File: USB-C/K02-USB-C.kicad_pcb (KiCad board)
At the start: 2 copper layers, 109.4 x 86.9 mm, 28 parts, among them SW1 SW_Push, SW10 SW_Push, SW11 SW_Push, SW12 SW_Push, SW13 SW_Push, SW14 SW_Push, SW15 SW_Push, SW16 SW_Push, SW17 SW_Push, SW2 SW_Push, SW3 SW_Push, SW4 SW_Push, SW5 SW_Push, SW6 SW_Push, SW7 SW_Push, SW8 SW_Push, SW9 SW_Push, U1 ProMicro-kbd

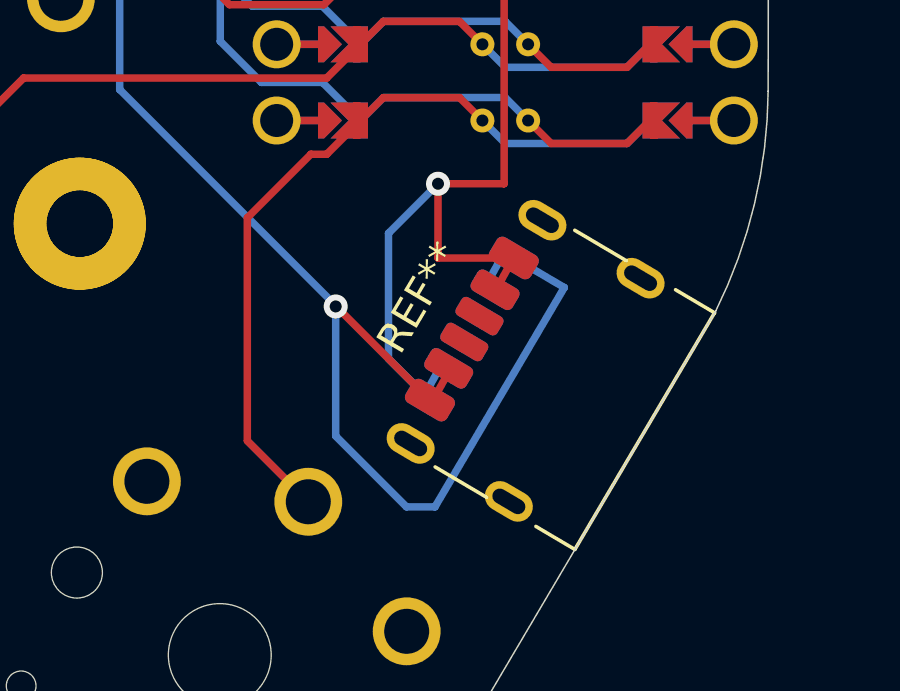
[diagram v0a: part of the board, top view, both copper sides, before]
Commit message: fixed
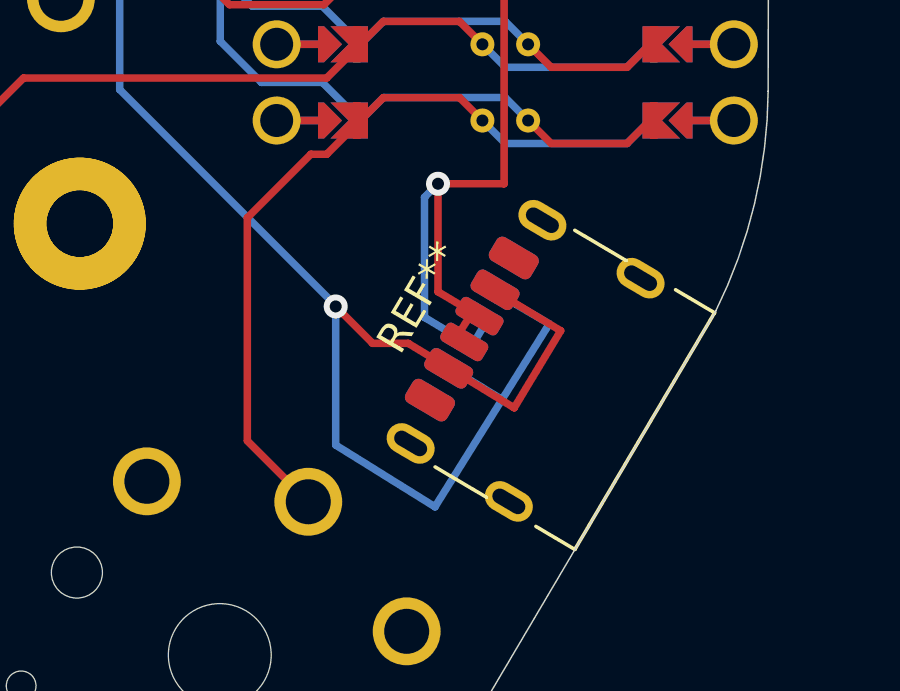
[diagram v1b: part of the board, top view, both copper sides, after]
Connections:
- REF** pad A12: Switch18 -> gnd (x2)
- REF** pad A5: (no net) -> Switch18
- REF** pad A9: Switch18 -> vcc (x2)
- REF** pad B12: vcc -> gnd (x2)
- REF** pad B5: (no net) -> Switch18
- REF** pad A5: gnd -> Switch18
- REF** pad B5: gnd -> Switch18
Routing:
- net Switch18: track 45.1 -> 38.3 mm
- net vcc: track 49.8 -> 44.3 mm
